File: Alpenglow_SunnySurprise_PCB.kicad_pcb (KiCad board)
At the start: 2 copper layers, 52.4 x 52.4 mm, 26 parts, among them SW1 SW_SPDT

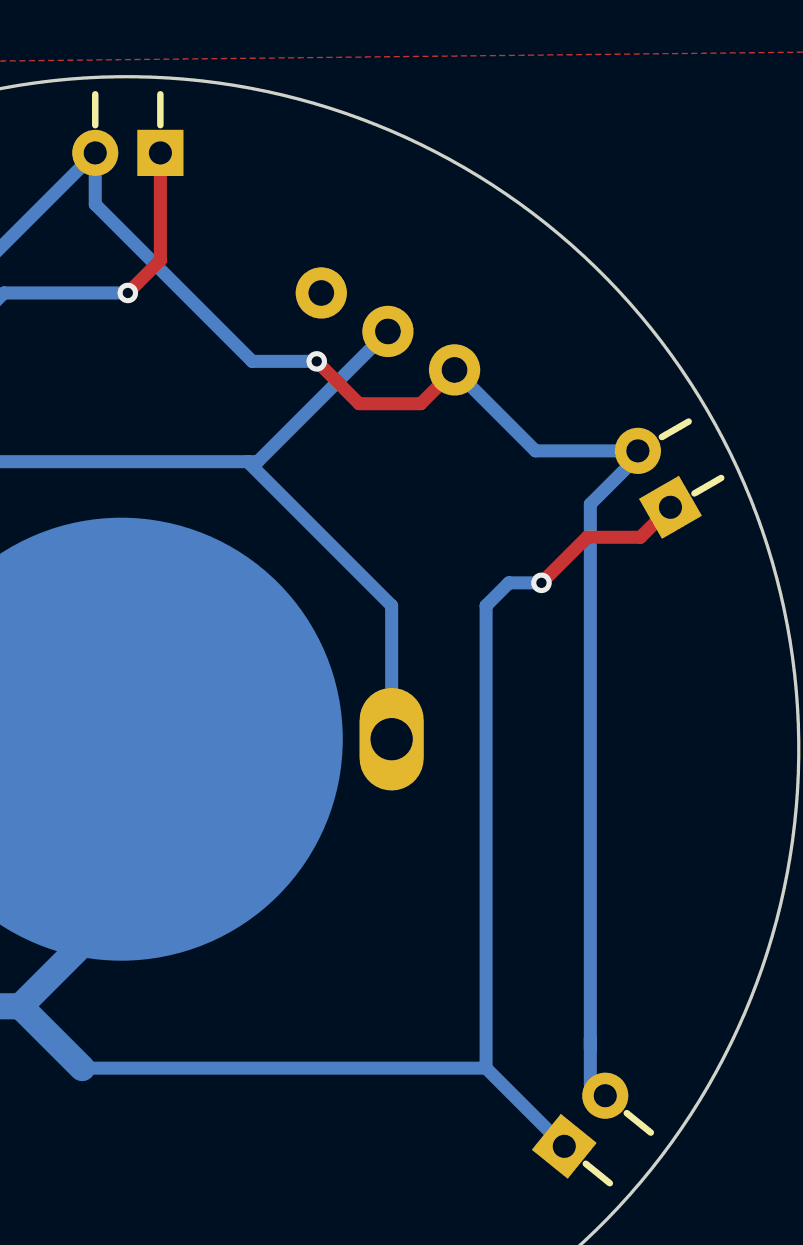
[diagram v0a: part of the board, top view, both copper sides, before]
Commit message: cleaned up short tracks, added fab notes, generated gerbers
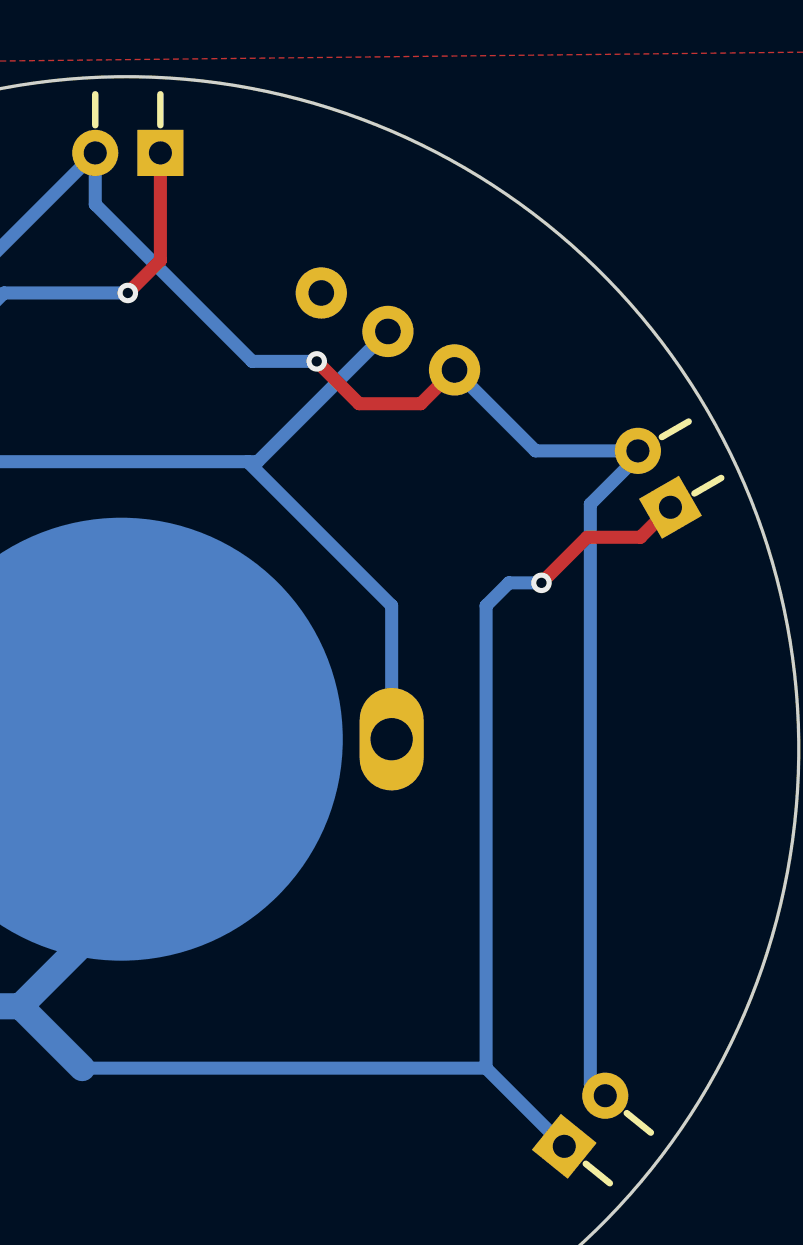
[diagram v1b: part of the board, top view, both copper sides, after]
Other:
- board text added: "Sunny Surprise Rev 2.0 PCB Specifications: 1. 1 oz Cu, FR-4 2. 2 layers 3. 0.063 inch / 1.6mm thick 4. Soldermask: Yellow, both sides 5. Silkscreen: Red, both sides 6. Finish: ENIG"
